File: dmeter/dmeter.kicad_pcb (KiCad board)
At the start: 2 copper layers, 185 x 72 mm, 104 parts, among them J1 INPUT, Q1 BC556, Q2 BC556, Q3 BC556, Q4 BC556, Q5 BC556, U1 TL072, U10 LM339, U2 TL072, U3 TL072, U4 TL072, U5 LM339, U6 LM339, U7 LM339, U8 LM339, U9 LM339

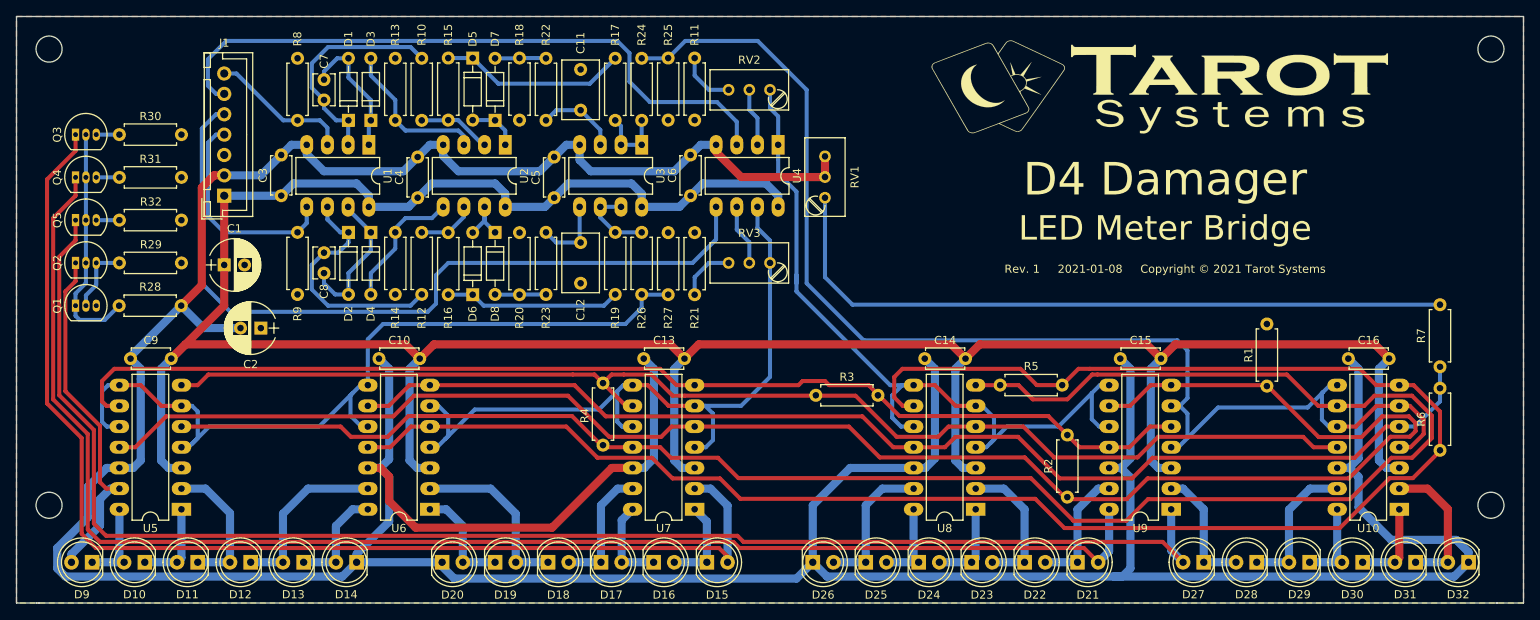
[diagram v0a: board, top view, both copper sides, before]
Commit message: Upgrade dmeter to Kicad 6
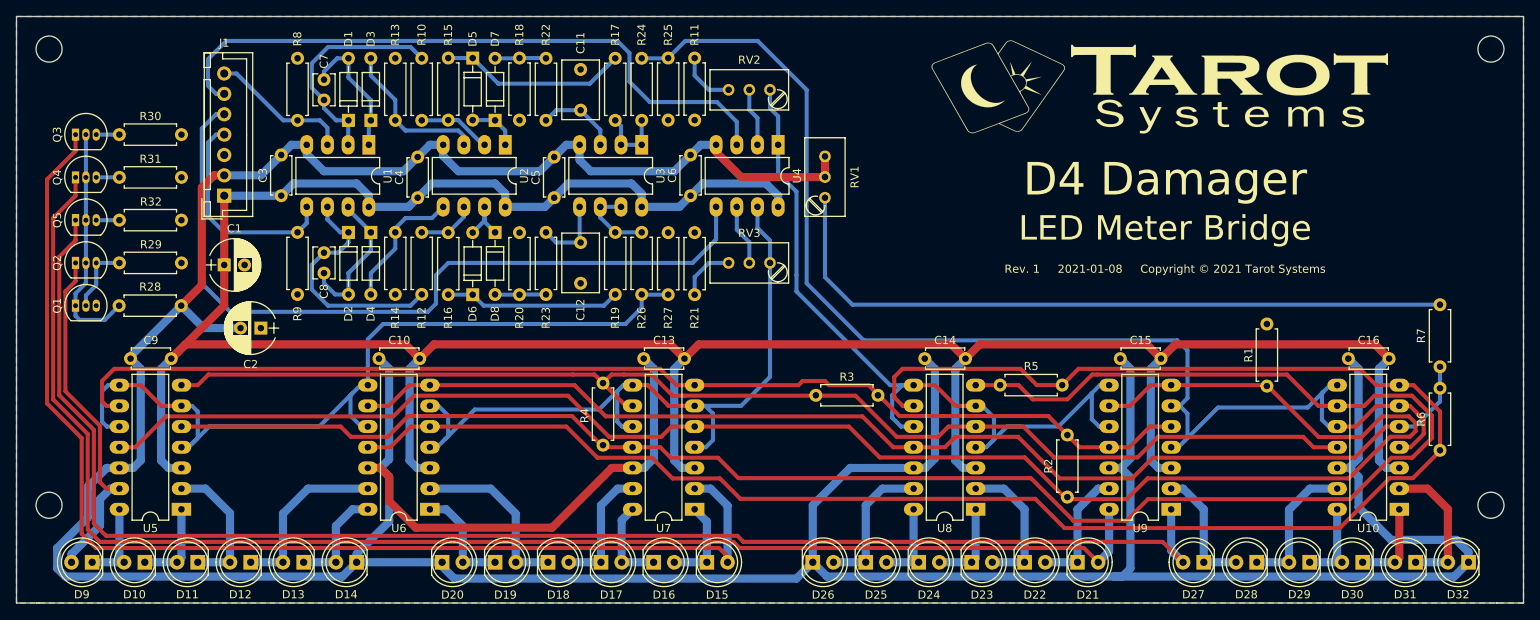
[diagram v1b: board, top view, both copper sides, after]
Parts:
- R24: value 30k -> 10k
- R26: value 10k -> 30k
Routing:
- net Net-(RV2-Pad1): track 95.2 -> 94.2 mm
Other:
- net class Default removed
- net class Power removed
